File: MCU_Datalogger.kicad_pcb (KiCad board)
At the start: 2 copper layers, 50 x 30.2 mm, 29 parts, among them J1 Conn_01x04_Pin, J2 Conn_01x09_Pin, J3 Conn_01x04_Pin, J4 Conn_02x03_Odd_Even, U1 24LC1025, U2 DS1337S_, U3 24LC1025, U4 ATMEGA328P-AU, Y1 32.768 KHz, Y2 16 MHz

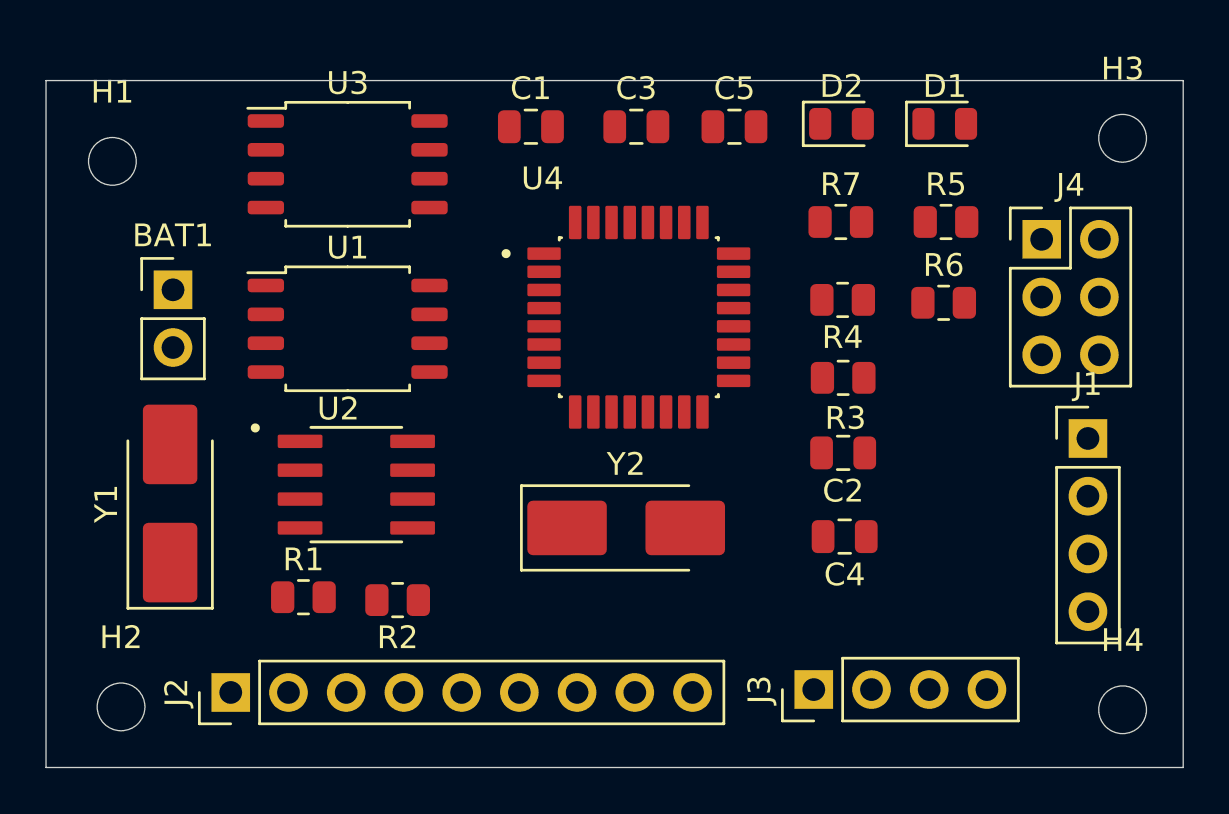
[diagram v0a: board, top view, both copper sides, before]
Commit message: Routing sans GND VCC complete.
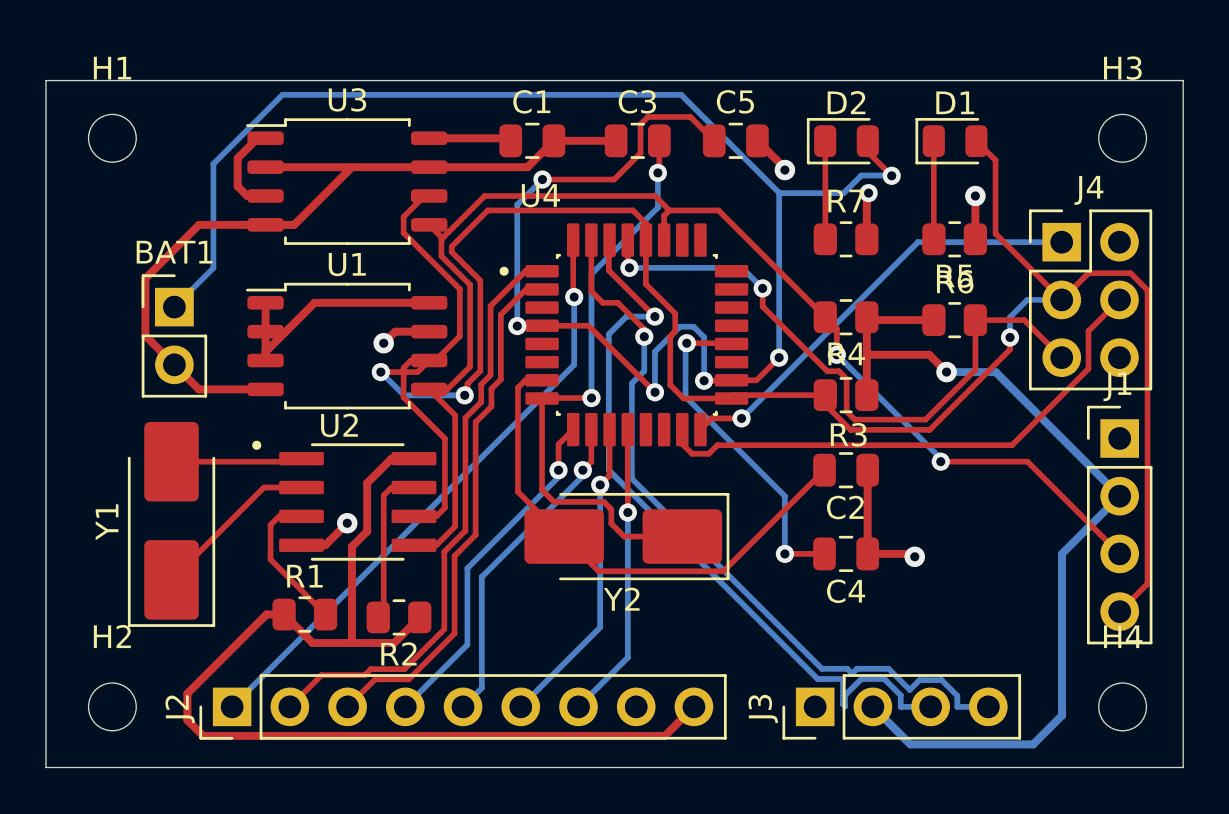
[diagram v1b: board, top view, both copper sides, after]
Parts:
- moved J1 1.40 mm to (183.0, 75.2)
- moved H1 1.02 mm to (138.7, 62.0)
- moved R6 0.90 mm to (175.7, 70.0)
- moved J4 0.89 mm to (180.5, 66.5)
- moved D1 0.89 mm to (175.8, 62.1)
- moved R5 0.85 mm to (175.7, 66.4), turned to 180 degrees
- moved R7 0.80 mm to (171.0, 66.4)
- moved D2 0.79 mm to (171.0, 62.1)
- moved U4 0.78 mm to (161.8, 70.6)
- moved R4 0.78 mm to (171.0, 69.8)
- moved C2 0.77 mm to (171.0, 76.6)
- moved R3 0.77 mm to (171.0, 73.3)
- moved BAT1 0.76 mm to (141.4, 69.4)
- moved J3 0.76 mm to (169.6, 87.0)
- moved R1 0.76 mm to (147.2, 82.9)
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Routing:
- net /VCC: track 0.00 -> 105.6 mm, vias 0 -> 1
- net /SCK: track 0.00 -> 99.7 mm, vias 0 -> 3
- net Net-(D2-A): track 0.00 -> 83.7 mm, vias 0 -> 6
- net /SDA: track 0.00 -> 57.1 mm, vias 0 -> 2
- net GND: track 0.00 -> 52.2 mm, vias 0 -> 6
- net /RX: track 0.00 -> 33.3 mm, vias 0 -> 1
- net /TX: track 0.00 -> 32.7 mm, vias 0 -> 1
- net /RESET: track 0.00 -> 28.1 mm, vias 0 -> 2
- net /D2: track 0.00 -> 26.8 mm, vias 0 -> 1
- net /D3: track 0.00 -> 26.2 mm
- net Net-(U4-PB7): track 0.00 -> 26.2 mm, vias 0 -> 2
- net /MOSI: track 0.00 -> 23.8 mm
- net /D4: track 0.00 -> 23.2 mm
- net Net-(U4-PB6): track 0.00 -> 22.6 mm
- net /MISO: track 0.00 -> 19.3 mm, vias 0 -> 1
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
